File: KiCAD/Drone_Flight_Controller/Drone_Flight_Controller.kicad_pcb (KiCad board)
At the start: 2 copper layers, 85 x 45 mm, 108 parts, among them J201 Conn_01x04, J205 XT60, J207 Conn_01x05, P601 USB_C_Plug_USB2.0, Q201 BC846C, Q202 BC856C, Q203 BC846C, Q204 BC856C, Q205 BC846C, Q206 BC856C, Q207 BC846C, Q208 BC856C, Q401 2N2222A, Q601 BC846C, Q602 BC846C, Q603 BC846C, Q604 BC846C, Q605 BC846C, Q606 BC846C, Q607 BC846C, SW1 SW_Push, U201 AS358, U202 AS358, U205 AS358, U301 DPS368, U302 BNO055, U303 ESP32-WROOM-32, U601 MCP2200-I-SO, U701 LM2576-3.3WT, Y601 CSTNE12M0GH5L000R0

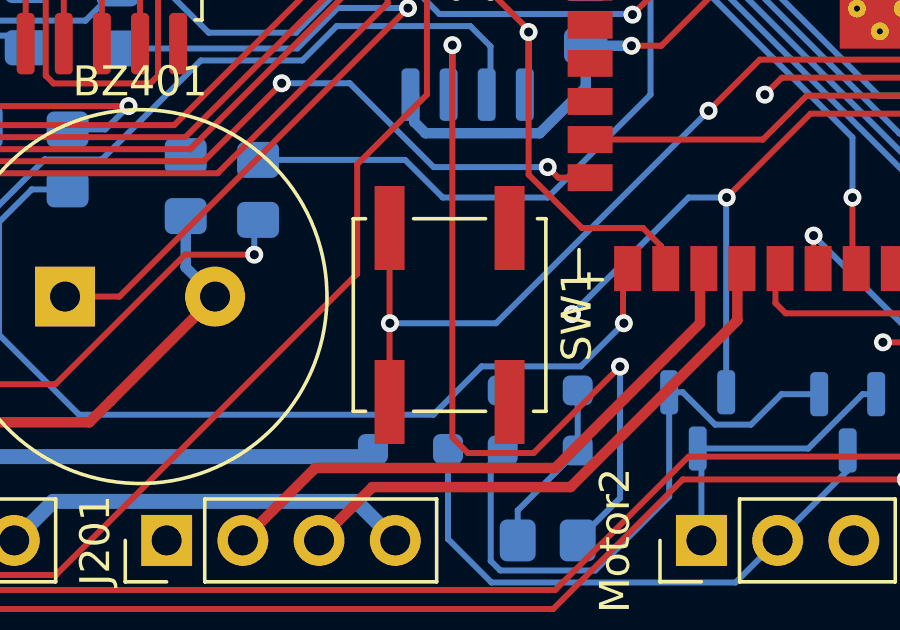
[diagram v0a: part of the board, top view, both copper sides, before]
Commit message: Fix Schematic PCB parity
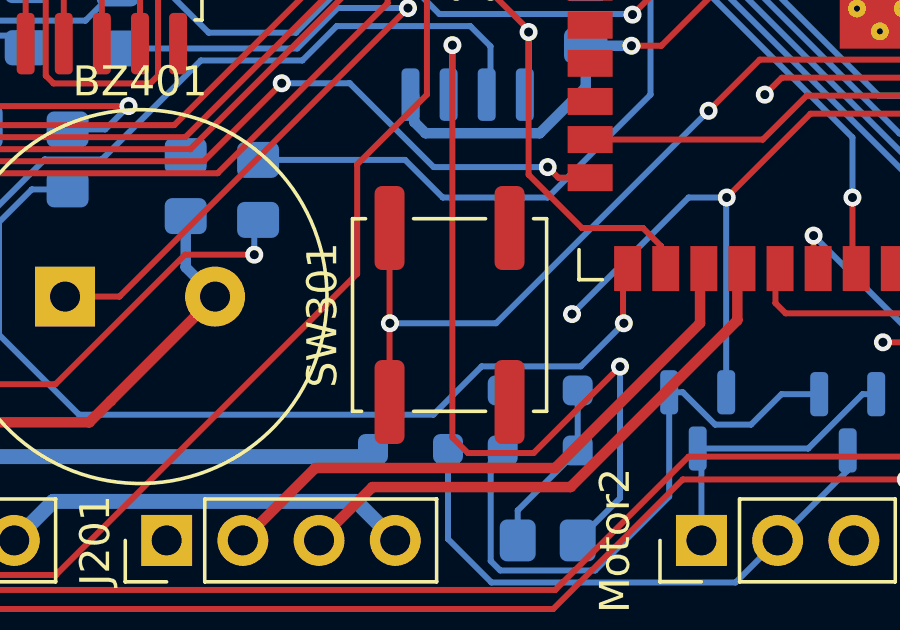
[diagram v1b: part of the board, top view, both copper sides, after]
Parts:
- removed SW1: SW_Push, Button_Switch_SMD:SW_Push_1P1T_NO_CK_KSC6xxJ
- added SW301: SW_Push, Button_Switch_SMD:SW_Push_1P1T_NO_CK_KSC6xxJ, F.Cu at (129.1, 107.5)
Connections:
- P601 pad A6: Net-(P601-D+) -> Net-(U601-D+)
- P601 pad A7: Net-(P601-D-) -> Net-(U601-D-)
- P601 pad B6: (no net) -> Net-(U601-D+)
- P601 pad B7: (no net) -> Net-(U601-D-)
- U601 pad 18: Net-(P601-D-) -> Net-(U601-D-)
- U601 pad 19: Net-(P601-D+) -> Net-(U601-D+)
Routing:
- net Net-(U601-D-): track 0.00 -> 20.3 mm
- net Net-(P601-D-): track 20.3 -> 0.00 mm
- net Net-(U601-D+): track 0.00 -> 20.0 mm
- net Net-(P601-D+): track 20.0 -> 0.00 mm
